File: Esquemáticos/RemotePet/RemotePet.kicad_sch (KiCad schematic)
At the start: 28 parts, among them U1 ESP32_DevKit_V1_DOIT, U2 xfw-hx711, U4 LM1117-3.3, U5 L7805, U6 GY-30

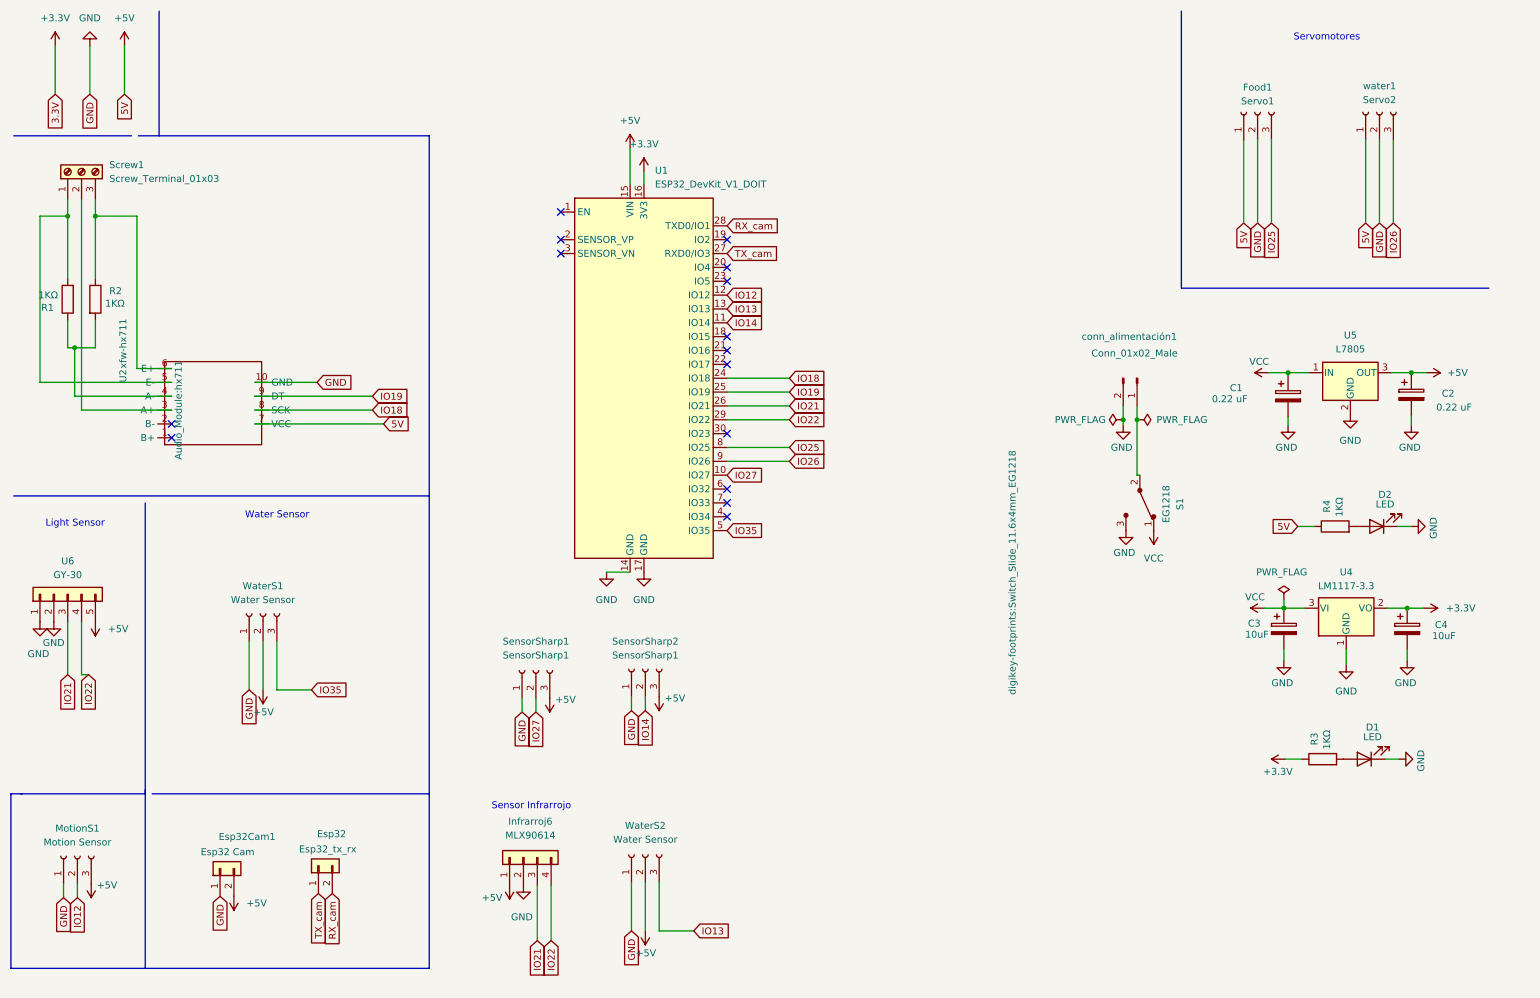
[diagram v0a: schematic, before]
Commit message: PCB 2.0
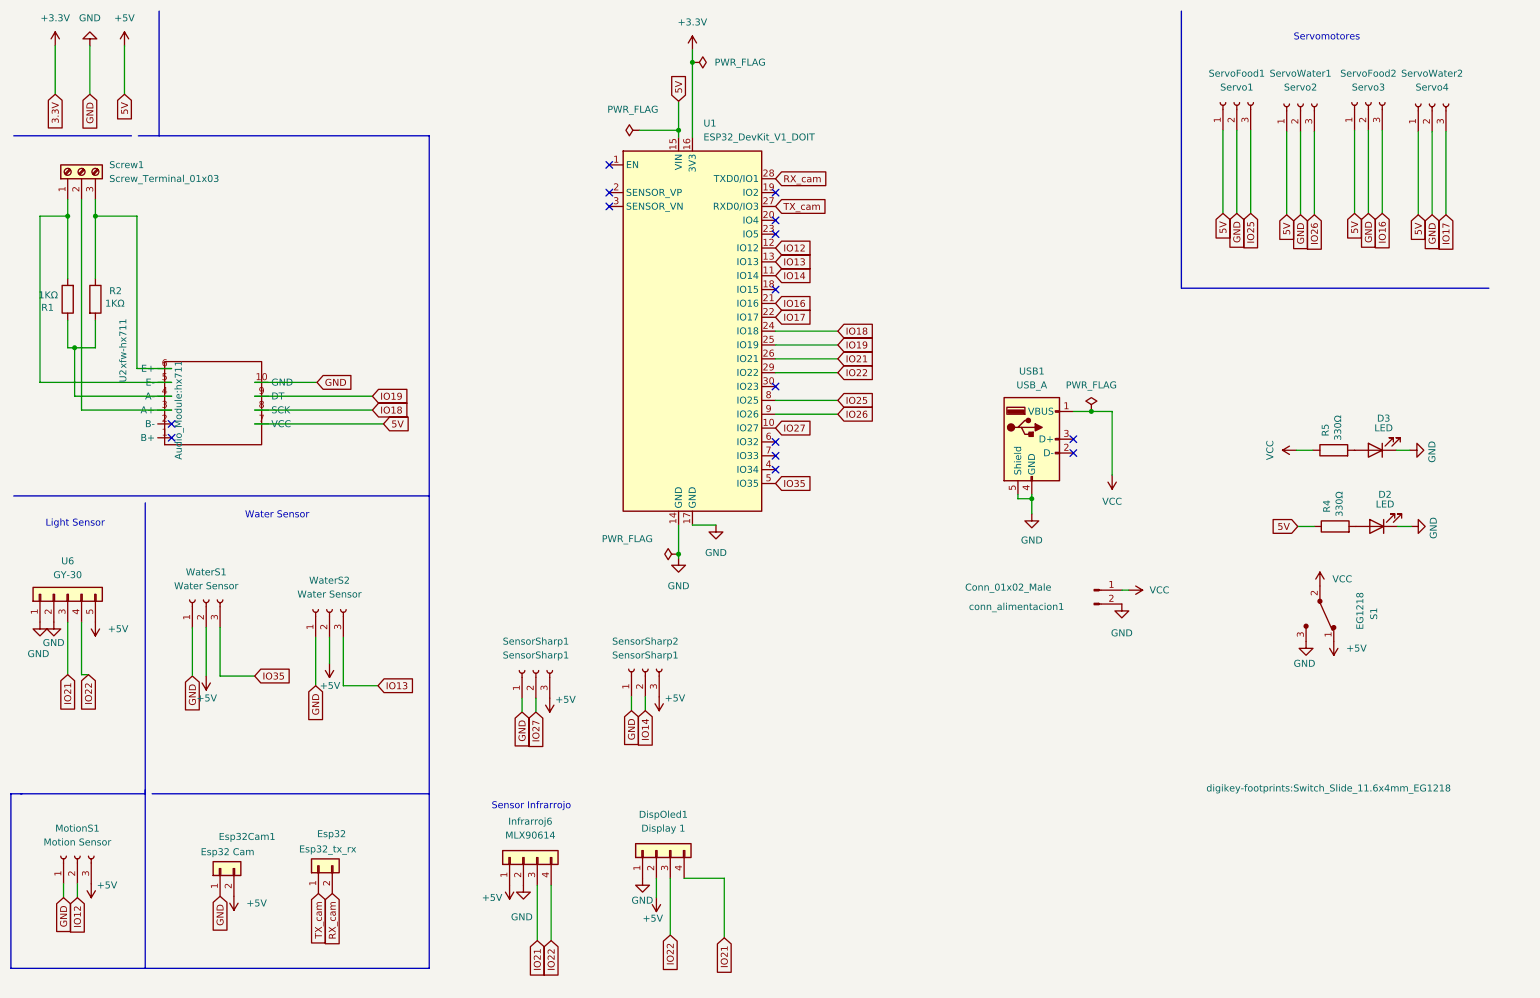
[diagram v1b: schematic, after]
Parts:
- removed C1, C2: 0.22 uF, Capacitor_THT:CP_Radial_D4.0mm_P2.00mm, symbol Device:C_Polarized
- removed C3, C4: 10uF, Capacitor_THT:CP_Radial_D4.0mm_P2.00mm, symbol Device:C_Polarized
- removed D1: LED, LED_THT:LED_D3.0mm_Clear, symbol Device:LED
- removed R3: 1KΩ, Resistor_THT:R_Axial_DIN0309_L9.0mm_D3.2mm_P12.70mm_Horizontal, symbol Device:R
- removed U4: LM1117-3.3, Package_TO_SOT_THT:TO-220-3_Vertical, symbol Regulator_Linear:LM1117-3.3
- removed U5: L7805, Package_TO_SOT_THT:TO-220-3_Vertical, symbol Regulator_Linear:L7805
- removed conn_alimentación1: Conn_01x02_Male, Connector_PinHeader_2.00mm:PinHeader_1x02_P2.00mm_Vertical, symbol Connector:Conn_01x02_Male
- added D3: LED, LED_SMD:LED_1210_3225Metric, symbol Device:LED
- added DispOled1: Display 1, Connector_PinSocket_2.54mm:PinSocket_1x04_P2.54mm_Vertical, symbol Connector_Generic:Conn_01x04
- added R5: 330Ω, Resistor_SMD:R_0805_2012Metric, symbol Device:R
- added ServoFood2: Servo3, Connector_PinSocket_2.54mm:PinSocket_1x03_P2.54mm_Vertical, symbol Connector:Conn_01x03_Female
- added ServoWater2: Servo4, Connector_PinSocket_2.54mm:PinSocket_1x03_P2.54mm_Vertical, symbol Connector:Conn_01x03_Female
- added USB1: USB_A, Connector_USB:USB_A_CONNFLY_DS1095-WNR0, symbol Connector:USB_A
- added conn_alimentacion1: Conn_01x02_Male, Connector_PinSocket_2.54mm:PinSocket_1x02_P2.54mm_Vertical, symbol Connector:Conn_01x02_Male
- D2: footprint LED_THT:LED_D3.0mm_Clear -> LED_SMD:LED_1210_3225Metric
- Esp32, Esp32Cam1: footprint Connector_PinSocket_2.00mm:PinSocket_1x02_P2.00mm_Vertical -> Connector_PinSocket_2.54mm:PinSocket_1x02_P2.54mm_Vertical
- Infrarroj6: footprint Connector_PinSocket_2.00mm:PinSocket_1x04_P2.00mm_Vertical -> Connector_PinSocket_2.54mm:PinSocket_1x04_P2.54mm_Vertical
- MotionS1, SensorSharp1, SensorSharp2, WaterS1, WaterS2: footprint Connector_PinSocket_2.00mm:PinSocket_1x03_P2.00mm_Vertical -> Connector_PinSocket_2.54mm:PinSocket_1x03_P2.54mm_Vertical
- R1, R2: footprint Resistor_THT:R_Axial_DIN0309_L9.0mm_D3.2mm_P12.70mm_Horizontal -> Resistor_SMD:R_0805_2012Metric
- R4: value 1KΩ -> 330Ω; footprint Resistor_THT:R_Axial_DIN0309_L9.0mm_D3.2mm_P12.70mm_Horizontal -> Resistor_SMD:R_0805_2012Metric
- Screw1: footprint TerminalBlock_4Ucon:TerminalBlock_4Ucon_1x03_P3.50mm_Vertical -> TerminalBlock:TerminalBlock_bornier-3_P5.08mm
- ServoFood1: renamed from Food1; footprint Connector_PinSocket_2.00mm:PinSocket_1x03_P2.00mm_Vertical -> Connector_PinSocket_2.54mm:PinSocket_1x03_P2.54mm_Vertical
- ServoWater1: renamed from water1; footprint Connector_PinSocket_2.00mm:PinSocket_1x03_P2.00mm_Vertical -> Connector_PinSocket_2.54mm:PinSocket_1x03_P2.54mm_Vertical
- U6: footprint Connector_PinSocket_2.00mm:PinSocket_1x05_P2.00mm_Vertical -> Connector_PinSocket_2.54mm:PinSocket_1x05_P2.54mm_Vertical
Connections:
- net +5V: now also S1.1, DispOled1.2 (Pin_2), ServoFood2.1 (Pin_1), ServoWater2.1 (Pin_1)
- net GND: now also D3.1 (K), DispOled1.1 (Pin_1), ServoFood2.2 (Pin_2), ServoWater2.2 (Pin_2), USB1.4 (GND), USB1.5 (Shield), conn_alimentacion1.2 (Pin_2)
- net IO21: now also DispOled1.4 (Pin_4)
- net IO22: now also DispOled1.3 (Pin_3)
- net VCC: now also S1.2, R5.1, USB1.1 (VBUS), conn_alimentacion1.1 (Pin_1); no longer S1.1
- net IO16: now reaches U1.21 (IO16)
- net IO16: now also ServoFood2.3 (Pin_3)
- net IO17: now reaches U1.22 (IO17)
- net IO17: now also ServoWater2.3 (Pin_3)
- new net: D3.2 (A), R5.2
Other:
- moved on the sheet: ServoFood1, ServoWater1, U1, WaterS1, WaterS2
